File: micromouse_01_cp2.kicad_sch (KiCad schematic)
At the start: 40 parts, among them IC1 ESP32-S3FH4R2, IC2 MPU-6500, IC3 AS5047P-ATSM, IC4 AS5047P-ATSM, IC5 DRV8835DSSR, J2 USB_B_Micro, M1 MK06-4.5, M2 MK06-4.5, SW2 SW_Push, U7 RTV-104DF333-S-40.000-TR

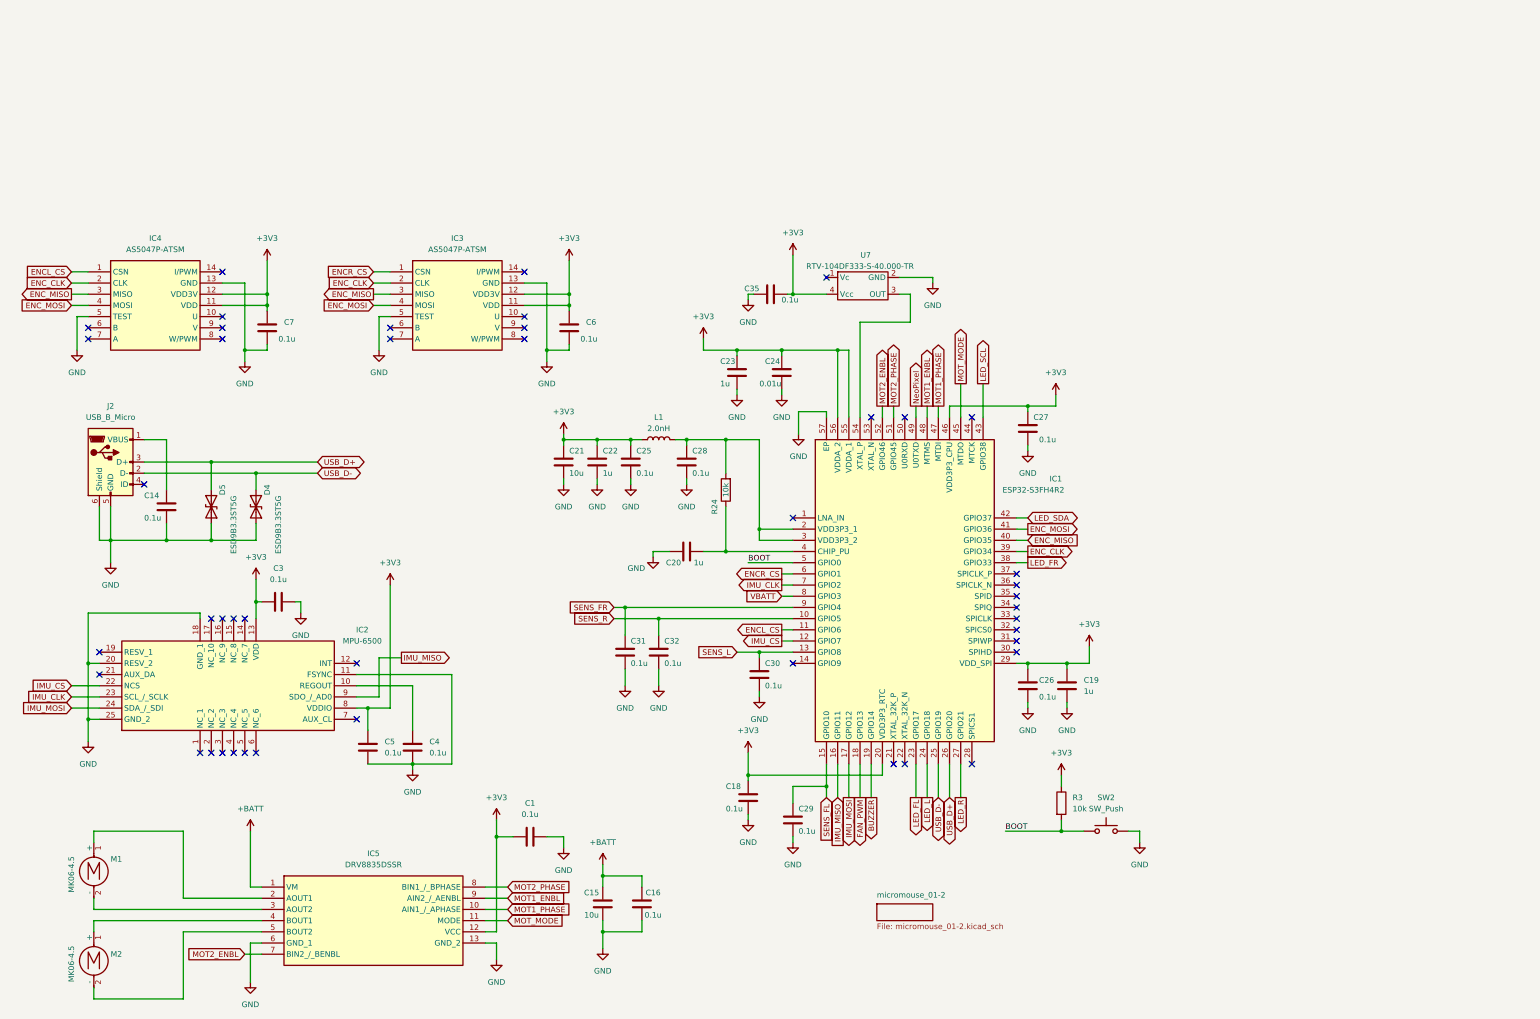
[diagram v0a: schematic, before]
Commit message: 仮変更
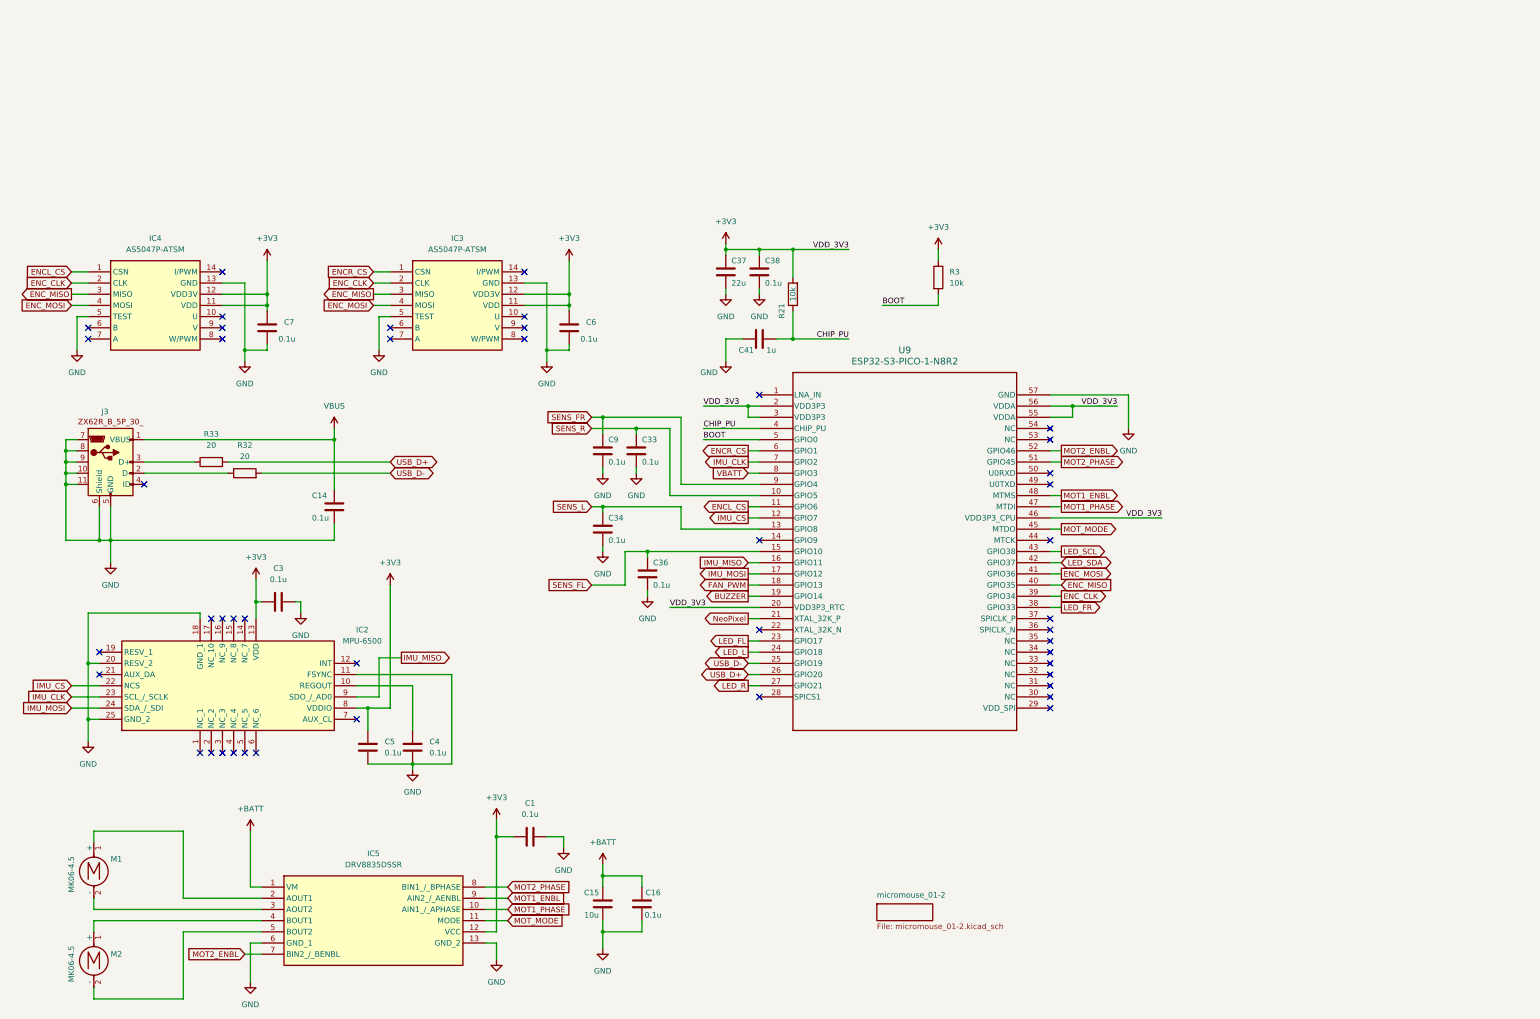
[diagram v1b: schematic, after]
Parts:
- removed C18, C25, C26, C27, C28, C29, C30, C31, C32, C35: 0.1u, Capacitor_SMD:C_0402_1005Metric, symbol Device:C
- removed C19, C20, C22, C23: 1u, Capacitor_SMD:C_0402_1005Metric, symbol Device:C
- removed C21: 10u, Capacitor_SMD:C_0603_1608Metric, symbol Device:C
- removed C24: 0.01u, Capacitor_SMD:C_0402_1005Metric, symbol Device:C
- removed D4, D5: ESD9B3.3ST5G, Diode_SMD:D_SOD-923, symbol Diode:ESD9B3.3ST5G
- removed IC1: ESP32-S3FH4R2, footprints:QFN40P700X700X90-57N-D, symbol ESP32-S3FH4R2:ESP32-S3FH4R2
- removed J2: USB_B_Micro, footprints:WURTH_614105150721, symbol Connector:USB_B_Micro
- removed L1: 2.0nH, Inductor_SMD:L_0402_1005Metric, symbol Device:L
- removed R24: 10k, Resistor_SMD:R_0402_1005Metric, symbol Device:R
- removed SW2: SW_Push, footprints:BOOT_PAD, symbol Switch:SW_Push
- removed U7: RTV-104DF333-S-40.000-TR, Crystal:Crystal_SMD_2016-4Pin_2.0x1.6mm, symbol RTV-104DF333-S-40.000-TR:RTV-104DF333-S-40.000-TR
- added C33, C34, C36, C38, C9: 0.1u, Capacitor_SMD:C_0402_1005Metric, symbol Device:C
- added C37: 22u, Capacitor_SMD:C_0603_1608Metric, symbol Device:C
- added C41: 1u, Capacitor_SMD:C_0402_1005Metric, symbol Device:C
- added J3: ~, footprints:ZX62R-B-5P_30_, symbol ZX62R_B_5P_30_:ZX62R_B_5P_30_
- added R21: 10k, Resistor_SMD:R_0402_1005Metric, symbol Device:R
- added R32, R33: 20, Resistor_SMD:R_0402_1005Metric, symbol Device:R
- added U9: ESP32-S3-PICO-1-N8R2, QFN56_7X7_EXP, symbol 2024-02-29_13-39-39:ESP32-S3-PICO-1-N8R2
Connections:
- net +3V3: now also C37.1, C38.1, R21.2, U9.2 (VDD3P3), U9.20 (VDD3P3_RTC), U9.3 (VDD3P3), U9.46 (VDD3P3_CPU), U9.55 (VDDA), U9.56 (VDDA)
- net BOOT: now also U9.5 (GPIO0)
- net BUZZER: now also U9.19 (GPIO14)
- net ENCL_CS: now also U9.11 (GPIO6)
- net ENCR_CS: now also U9.6 (GPIO1)
- net ENC_CLK: now also U9.39 (GPIO34)
- net ENC_MISO: now also U9.40 (GPIO35)
- net ENC_MOSI: now also U9.41 (GPIO36)
- net FAN_PWM: now also U9.18 (GPIO13)
- net GND: now also C33.2, C34.2, C36.2, C37.2, C38.2, C41.1, C9.2, J3.10, J3.11, J3.5 (GND), J3.6 (Shield), J3.7, J3.8, J3.9, U9.57 (GND)
- net IMU_CLK: now also U9.7 (GPIO2)
- net IMU_CS: now also U9.12 (GPIO7)
- net IMU_MISO: now also U9.16 (GPIO11)
- net IMU_MOSI: now also U9.17 (GPIO12)
- net LED_FL: now also U9.23 (GPIO17)
- net LED_FR: now also U9.38 (GPIO33)
- net LED_L: now also U9.24 (GPIO18)
- net LED_R: now also U9.27 (GPIO21)
- net LED_SCL: now also U9.43 (GPIO38)
- net LED_SDA: now also U9.42 (GPIO37)
- net MOT1_ENBL: now also U9.48 (MTMS)
- net MOT1_PHASE: now also U9.47 (MTDI)
- net MOT2_ENBL: now also U9.52 (GPIO46)
- net MOT2_PHASE: now also U9.51 (GPIO45)
- net MOT_MODE: now also U9.45 (MTDO)
- net NeoPixel: now also U9.21 (XTAL_32K_P)
- net SENS_FL: now also C36.1, U9.15 (GPIO10)
- net SENS_FR: now also C9.1, U9.9 (GPIO4)
- net SENS_L: now also C34.1, U9.13 (GPIO8)
- net SENS_R: now also C33.1, U9.10 (GPIO5)
- net USB_D+: now also R33.2, U9.26 (GPIO20)
- net USB_D-: now also R32.2, U9.25 (GPIO19)
- net VBATT: now also U9.8 (GPIO3)
- net VBUS: now reaches C14.1
- net VBUS: now also J3.1 (VBUS)
- new net: J3.2 (D-), R32.1
- new net: J3.3 (D+), R33.1
- new net CHIP_PU: C41.2, R21.1, U9.4 (CHIP_PU)
- no-connect marks 44 -> 45
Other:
- moved on the sheet: C14, R3

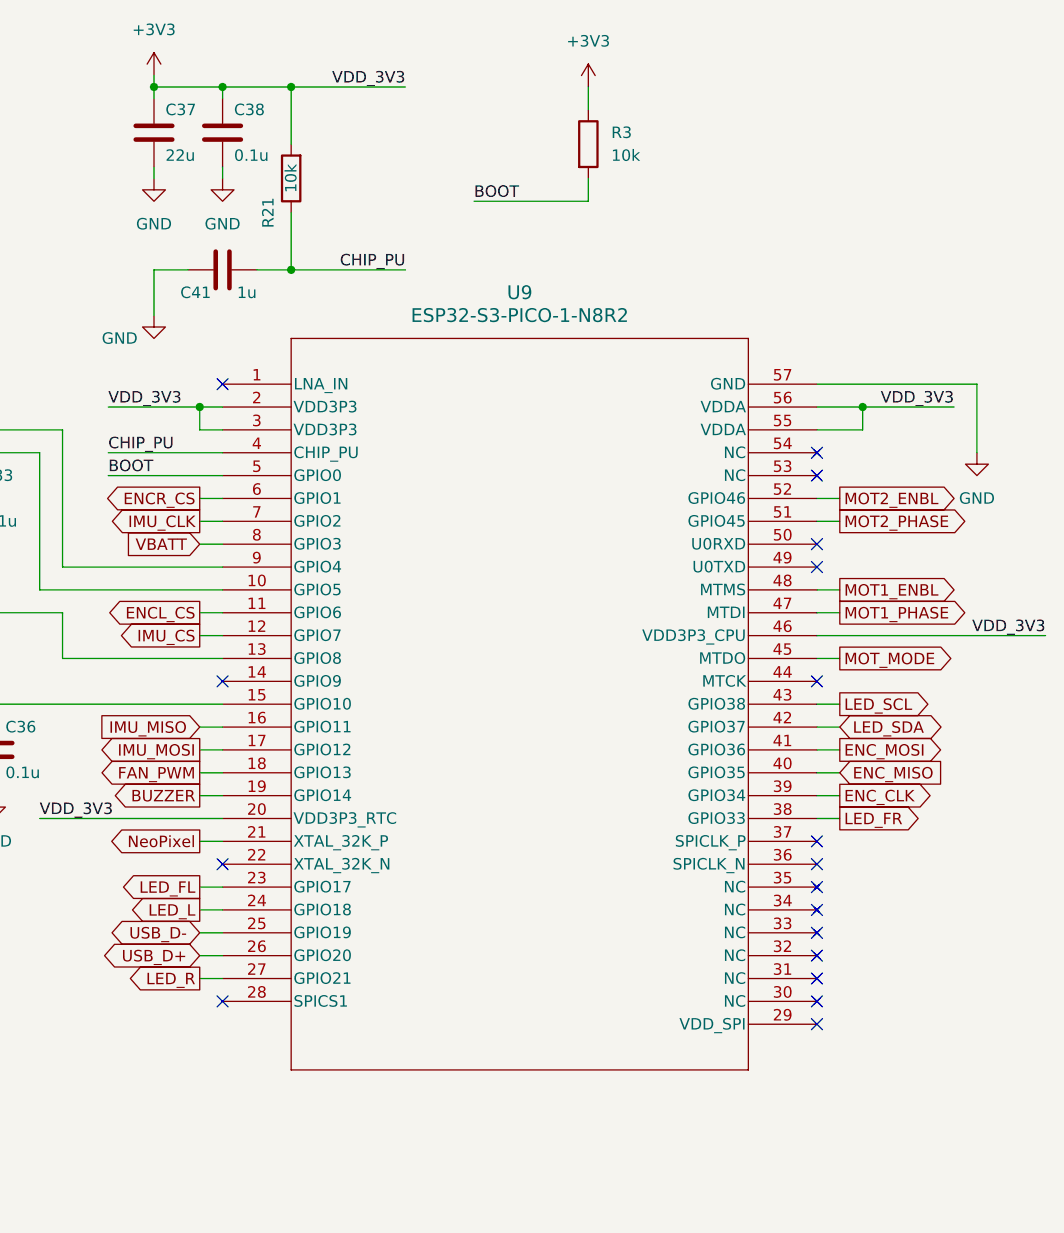
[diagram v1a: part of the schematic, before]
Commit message: [update]けっこう線引いた
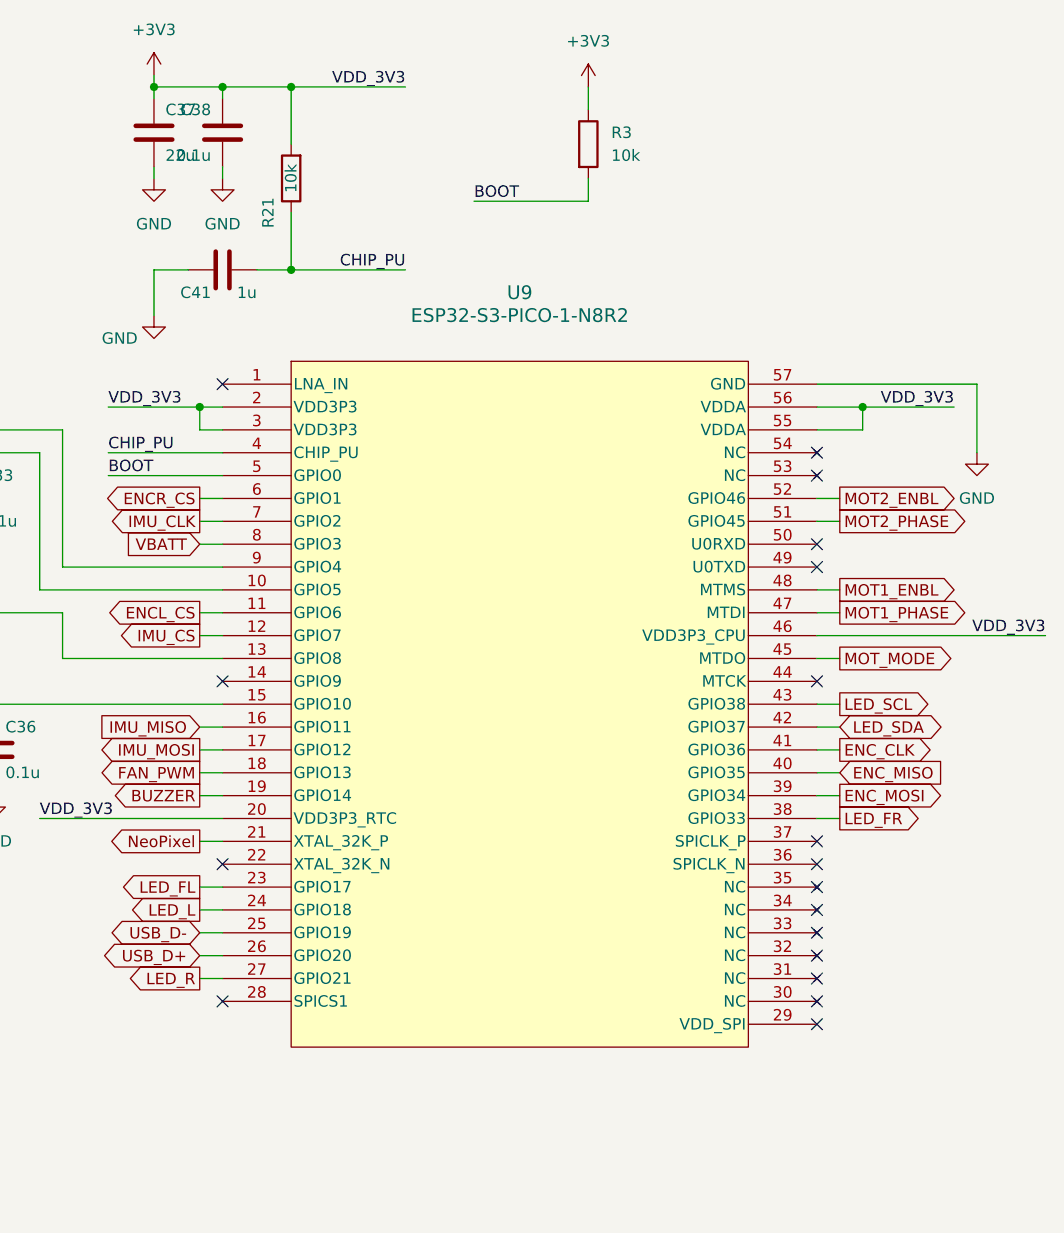
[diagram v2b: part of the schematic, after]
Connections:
- net ENC_CLK: now also U9.41 (GPIO36); no longer U9.39 (GPIO34)
- net ENC_MOSI: now also U9.39 (GPIO34); no longer U9.41 (GPIO36)
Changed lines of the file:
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@@
+    )
+  )
+  (global_label "ENC_MOSI" (shape output) (at 256.54 101.6 0) (fields_autoplaced)
+    (effects (font (size 1.27 1.27)) (justify left))
+    (property "Intersheetrefs" "${INTERSHEET_REFS}" (at 268.8385 101.6 0)
+      (effects (font (size 1.27 1.27)) (justify left) hide)
     )
   )
@@
     )
   )
+  (global_label "ENC_CLK" (shape output) (at 256.54 96.52 0) (fields_autoplaced)
+    (effects (font (size 1.27 1.27)) (justify left))
+    (property "Intersheetrefs" "${INTERSHEET_REFS}" (at 267.8104 96.52 0)
+      (effects (font (size 1.27 1.27)) (justify left) hide)
+    )
+  )
   (global_label "ENC_MISO" (shape output) (at 100.33 33.02 180) (fields_autoplaced)
     (effects (font (size 1.27 1.27)) (justify right))
@@
     )
   )
-  (global_label "ENC_CLK" (shape output) (at 256.54 101.6 0) (fields_autoplaced)
-    (effects (font (size 1.27 1.27)) (justify left))
-    (property "Intersheetrefs" "${INTERSHEET_REFS}" (at 267.8104 101.6 0)
-      (effects (font (size 1.27 1.27)) (justify left) hide)
-    )
-  )
   (global_label "IMU_MOSI" (shape input) (at 31.75 127 180) (fields_autoplaced)
     (effects (font (size 1.27 1.27)) (justify right))
     (property "Intersheetrefs" "${INTERSHEET_REFS}" (at 19.8143 127 0)
       (effects (font (size 1.27 1.27)) (justify right) hide)
-    )
-  )
-  (global_label "ENC_MOSI" (shape output) (at 256.54 96.52 0) (fields_autoplaced)
-    (effects (font (size 1.27 1.27)) (justify left))
-    (property "Intersheetrefs" "${INTERSHEET_REFS}" (at 268.8385 96.52 0)
-      (effects (font (size 1.27 1.27)) (justify left) hide)
     )
   )
@@
     )
   )
-  (symbol (lib_id "Device:C") (at 187.96 27.94 0) (unit 1)
+  (symbol (lib_id "Device:C") (at 187.96 27.94 0) (mirror y) (unit 1)
     (in_bom yes) (on_board yes) (dnp no)
-    (property "Reference" "C38" (at 189.23 25.4 0)
-      (effects (font (size 1.27 1.27)) (justify left))
-    )
-    (property "Value" "0.1u" (at 189.23 30.48 0)
-      (effects (font (size 1.27 1.27)) (justify left))
-    )
-    (property "Footprint" "Capacitor_SMD:C_0402_1005Metric" (at 188.9252 31.75 0)
-      (effects (font (size 1.27 1.27)) hide)
-    )
+    (property "Reference" "C38" (at 186.69 25.4 0)
+      (effects (font (size 1.27 1.27)) (justify left))
+    )
+    (property "Value" "0.1u" (at 186.69 30.48 0)
+      (effects (font (size 1.27 1.27)) (justify left))
+    )
+    (property "Footprint" "Capacitor_SMD:C_0402_1005Metric" (at 186.9948 31.75 0)
+      (effects (font (size 1.27 1.27)) hide)
+    )
